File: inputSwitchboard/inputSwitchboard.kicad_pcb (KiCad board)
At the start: 2 copper layers, 65 parts, among them J1 DATA, J10 BOOTSEL, J11 RESET, J12 DEBUG, J2 POWER, J3 INPUT SEL, J4 OUTPUT SEL, J5 INT CTRL, J6 EXT CTRL, J7 NES, J8 GPIO, U1 AMS1117-3.3, U10 W25Q128JVS, U2 RP2040, U3 CH442E, U4 CH442E, U5 CH442E, U6 CH442E, U7 CH442E, U8 CH442E, U9 TXS0108EPW, Y1 ABM8-272-T3

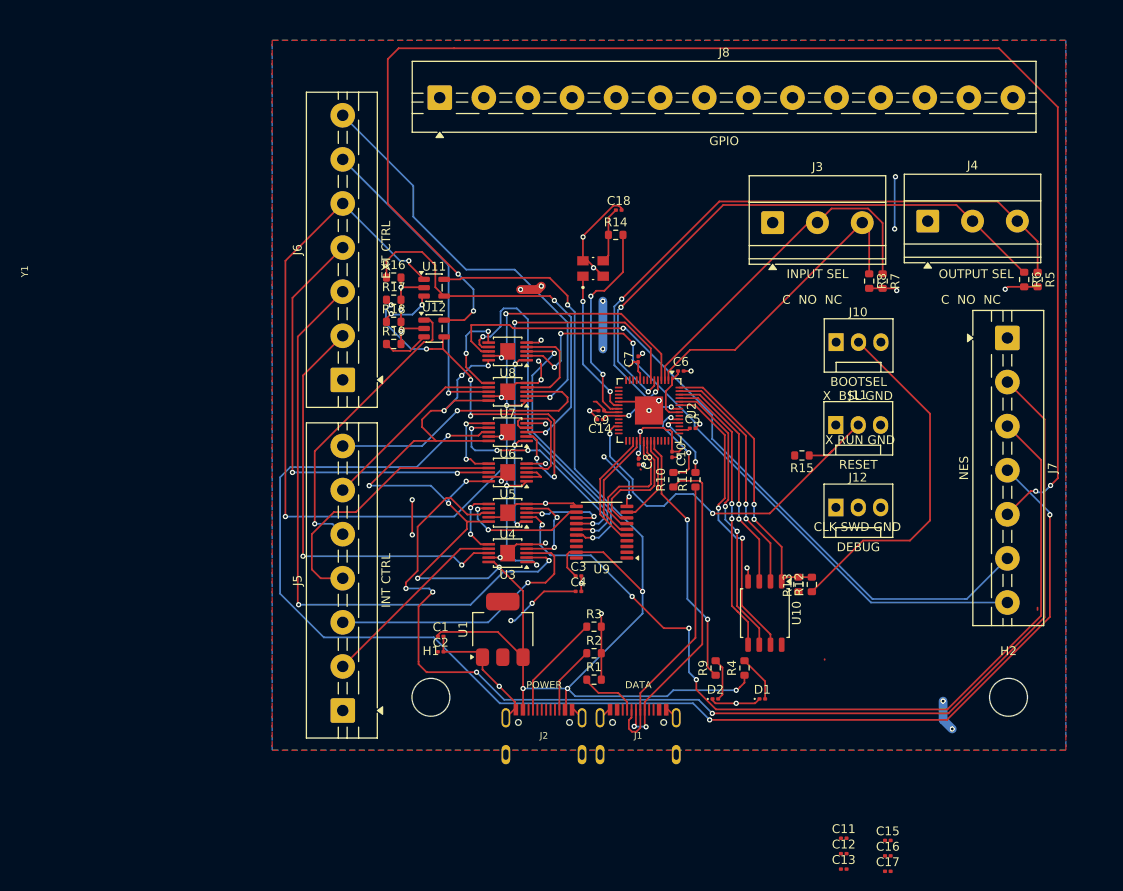
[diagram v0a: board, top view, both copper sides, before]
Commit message: fixed more stuff and polished routing
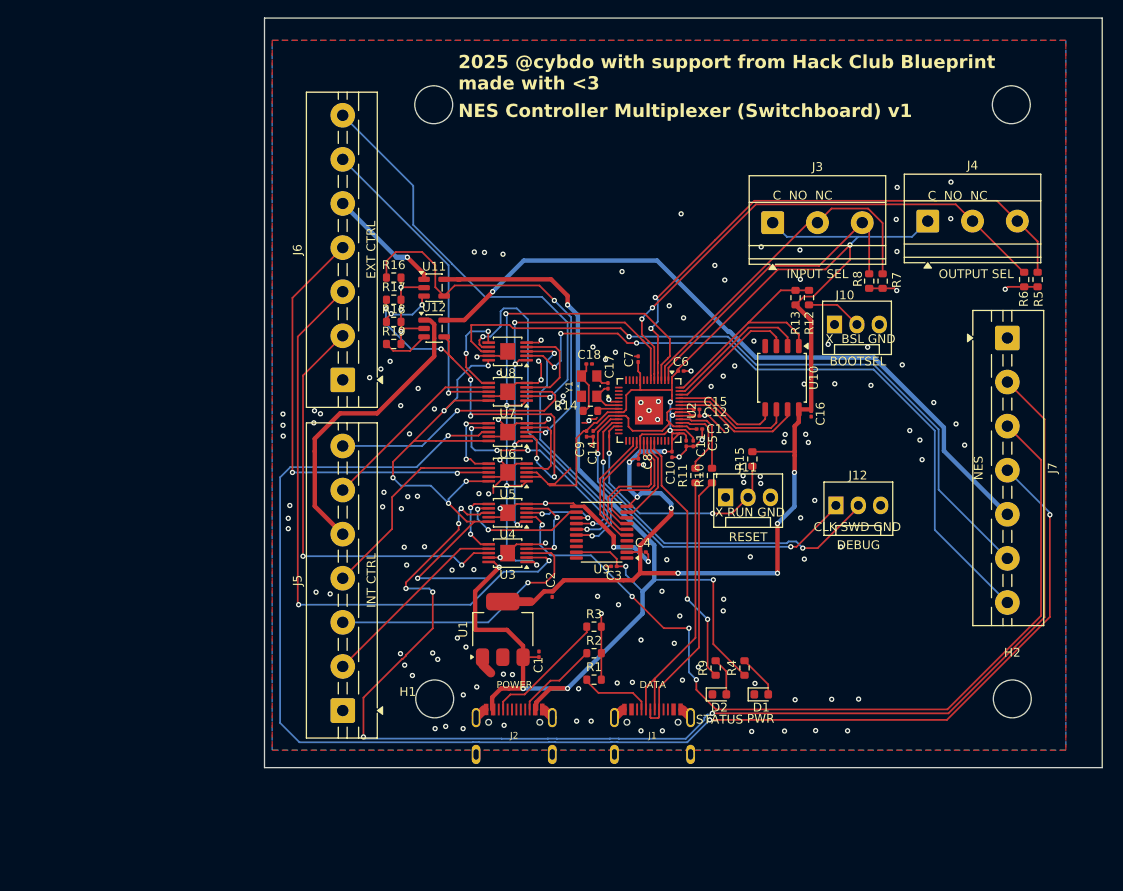
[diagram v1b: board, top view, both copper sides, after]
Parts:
- removed J8: GPIO, TerminalBlock:TerminalBlock_MaiXu_MX126-5.0-14P_1x14_P5.00mm
- added ?: , , F.Cu at (140.3, 39.3)
- added ?: , , F.Cu at (74.8, 39.3)
- added G***: LOGO, imports:rickroll, F.Cu at (93.8, 74.5)
- D1, D2: footprint LED_SMD:LED_0201_0603Metric -> LED_SMD:LED_0603_1608Metric
- moved C17 63.5 mm to (94.6, 71.2), turned to 90 degrees
- moved C15 53.5 mm to (104.6, 73.8)
- moved C13 52.5 mm to (104.9, 76.1)
- moved C12 52.4 mm to (104.6, 74.6)
- moved C16 50.9 mm to (117.6, 74.3), turned to -90 degrees
- moved C11 48.2 mm to (103.5, 77.7), turned to -90 degrees
- moved R12 32.5 mm to (117.4, 61.2)
- moved R13 32.5 mm to (115.8, 61.2)
- moved U10 26.8 mm to (114.3, 70.3)
- moved R14 20.2 mm to (92.6, 74.0)
- moved C18 17.8 mm to (92.4, 68.7)
- moved J11 14.9 mm to (107.9, 83.8)
- moved C2 14.2 mm to (88.2, 94.8), turned to -90 degrees
- moved Y1 13.3 mm to (92.4, 71.2), turned to 180 degrees
- moved C1 11.3 mm to (86.8, 101.6), turned to 90 degrees
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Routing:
- net +3V3: track 60.6 -> 217.7 mm
- net PROC-NES-4-VCC: track 165.2 -> 80.2 mm, vias 4 -> 1
- net CTRL-EXT-4-VCC: track 78.1 -> 13.1 mm, vias 2 -> 1
- net Net-(J12-Pin_2): track 0.00 -> 42.0 mm, vias 0 -> 2
- net Net-(J12-Pin_1): track 0.00 -> 41.3 mm, vias 0 -> 2
- net Net-(J10-Pin_2): track 40.3 -> 6.36 mm
- net XOUT: track 23.6 -> 2.14 mm, vias 2 -> 0
- net NAND-SD0: track 32.4 -> 12.3 mm, vias 2 -> 0
- net NAND-SCLK: track 32.8 -> 14.0 mm, vias 2 -> 0
- net NAND-SD3: track 33.5 -> 15.0 mm, vias 2 -> 0
- net GND: track 129.0 -> 111.7 mm, vias 37 -> 155
- net RUN: track 44.1 -> 29.2 mm
- net PROC-NES-1-CLK: track 136.1 -> 149.7 mm, vias 4 -> 6
- net XIN: track 16.6 -> 4.52 mm, vias 2 -> 0
- net NAND-SD2: track 26.3 -> 15.3 mm, vias 2 -> 0
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- added copper zone on F.Cu, net GND
- removed copper zone on F.Cu, net +3V3
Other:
- board outline added: 95 x 85 mm
- board text added: "2025 @cybdo with support from Hack Club Blueprint made with <3"
- board text added: "NES Controller Multiplexer (Switchboard) v1"
- board text added: "PWR"
- board text added: "STATUS"
